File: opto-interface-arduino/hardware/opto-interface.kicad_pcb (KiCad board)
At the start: 2 copper layers, 24 parts, among them P1 CONN_02X06, P2 CONN_01X06, U1 max889, U2 LM7805, U3 LM7905

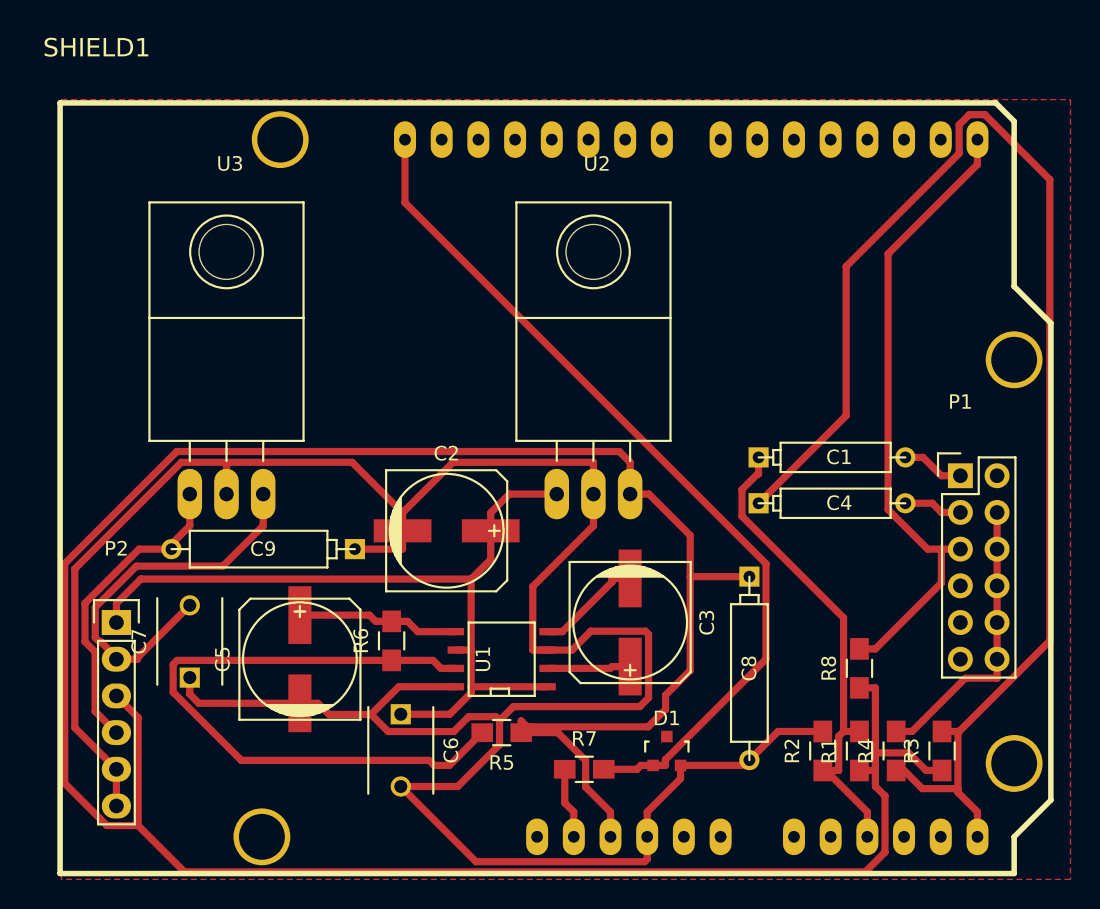
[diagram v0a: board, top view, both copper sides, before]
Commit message: Complete v 0.1 layout
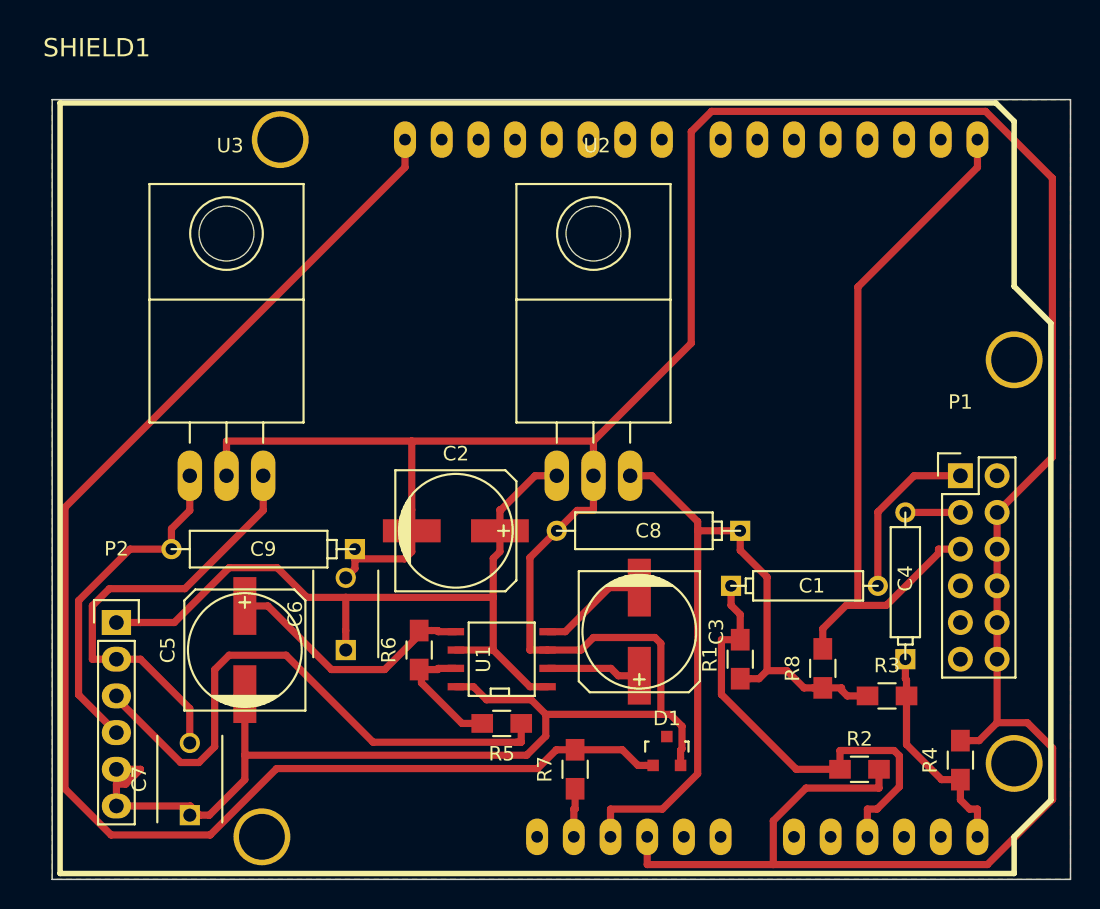
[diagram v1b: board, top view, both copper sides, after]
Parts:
- moved C8 11.8 mm to (189.2, 81.3), turned to 180 degrees
- moved R1 10.4 mm to (195.6, 90.2)
- moved C7 9.53 mm to (157.5, 101.0)
- moved C1 9.09 mm to (200.0, 85.1)
- moved C4 7.65 mm to (207.0, 85.1), turned to 90 degrees
- moved C6 5.85 mm to (168.3, 89.5), turned to 90 degrees
- moved R3 5.39 mm to (205.7, 92.7), turned to 0 degrees
- moved R4 4.49 mm to (210.8, 97.2)
- moved C5 3.86 mm to (161.3, 89.5)
- moved R2 2.84 mm to (203.8, 97.8), turned to 0 degrees
- moved R8 2.54 mm to (201.3, 90.8)
- moved R6 2.01 mm to (173.4, 89.5)
- moved U2 1.27 mm to (185.4, 77.5)
- moved U3 1.27 mm to (160.0, 77.5)
- moved C3 0.90 mm to (188.6, 88.3)
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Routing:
- net +5V: track 193.4 -> 95.7 mm
- net GND: track 204.3 -> 284.4 mm
- net Net-(C4-Pad1): track 95.0 -> 15.4 mm
- net Net-(D1-Pad1): track 60.9 -> 99.6 mm
- net Net-(R5-Pad2): track 46.3 -> 8.90 mm
- net Net-(C1-Pad2): track 4.34 -> 11.9 mm
- net Net-(C5-Pad1): track 11.3 -> 18.1 mm
- net Net-(P1-Pad5): track 44.2 -> 49.0 mm
- net -12V: track 27.1 -> 31.2 mm
- net +12V: track 56.5 -> 54.4 mm
- net -5V: track 21.7 -> 23.7 mm
- net +3V3: track 4.93 -> 3.41 mm
- net Net-(C1-Pad1): track 33.1 -> 31.9 mm
- net Net-(C3-Pad1): track 5.77 -> 6.56 mm
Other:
- board outline added: 70.5 x 54 mm
- net class Default: clearance 0.2 -> 0.4
- rule trace_clearance: 0.2 -> 0.4
